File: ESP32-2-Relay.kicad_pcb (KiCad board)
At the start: 2 copper layers, 98 x 94 mm, 44 parts, among them J1 Relay-1, J2 Relay-2, J3 USB_C_Receptacle_USB2.0, K1 SRD-05VDC-SL-C, K2 SRD-05VDC-SL-C, Q1 BC857, Q2 BC857, Q3 BC847W, Q4 BC847W, SW3 SW_Push, SW4 SW_Push, U1 AMS1117-3.3, U4 ESP32-WROOM-32, U5 PC817, U6 PC817, U7 USBLC6-2SC6, U8 CP2102N-Axx-xQFN28

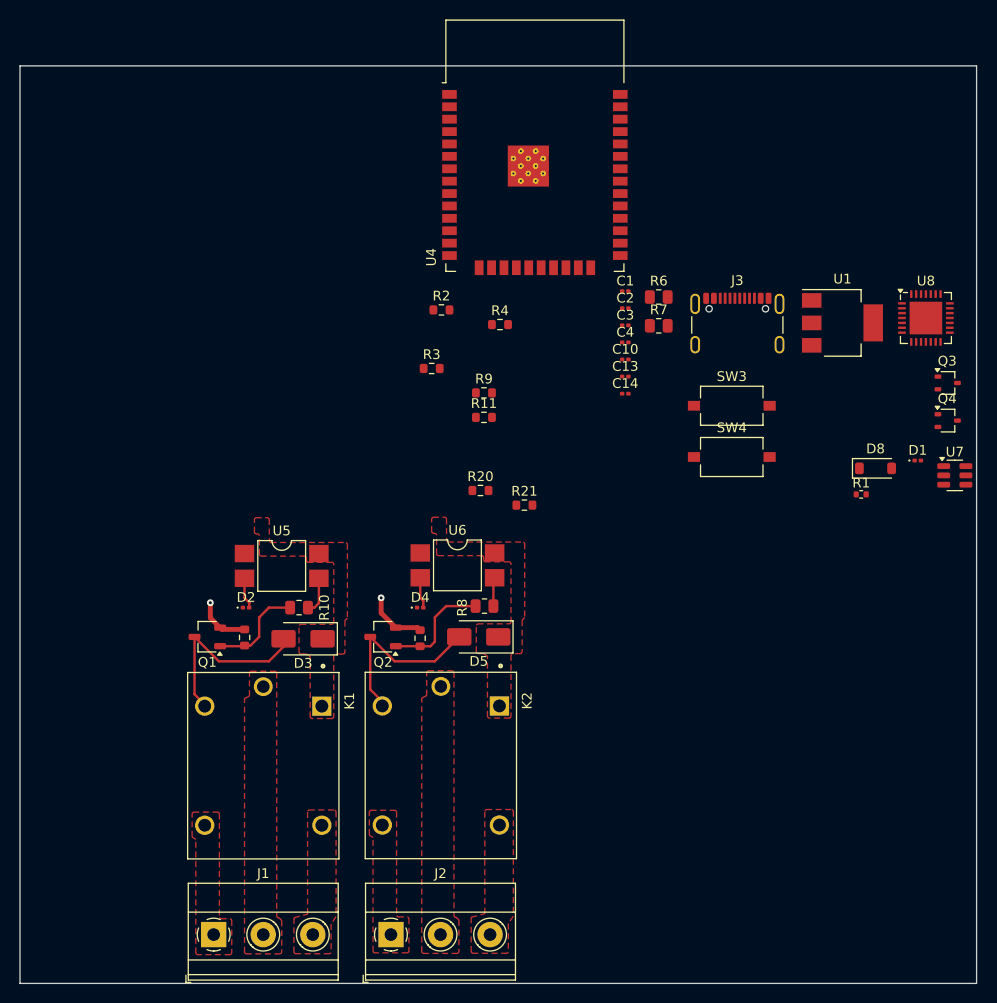
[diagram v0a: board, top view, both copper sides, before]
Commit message: 17h
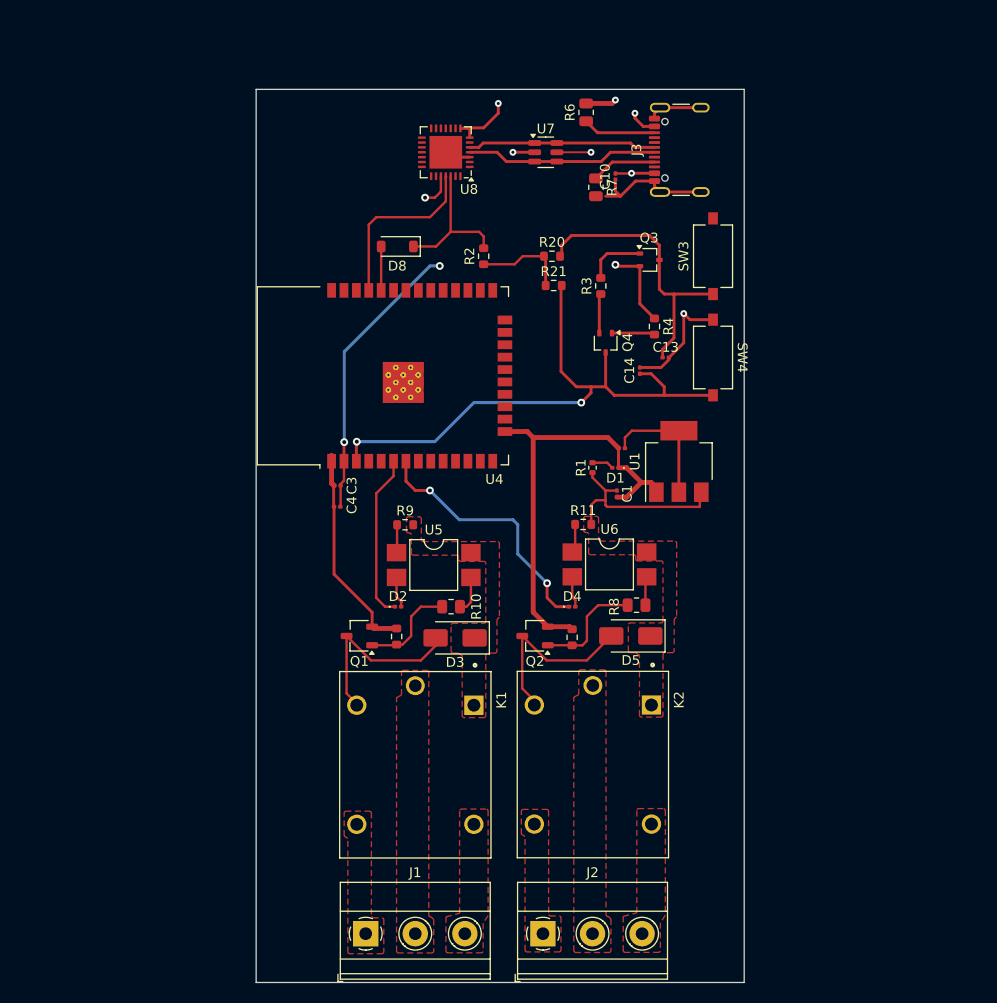
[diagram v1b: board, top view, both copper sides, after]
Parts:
- moved D8 54.0 mm to (173.2, 73.5), turned to 180 degrees
- moved U7 53.4 mm to (188.4, 63.9)
- moved U8 52.0 mm to (178.1, 63.9), turned to 180 degrees
- moved Q4 35.9 mm to (194.5, 83.4), turned to -90 degrees
- moved C4 34.0 mm to (167.0, 100.2), turned to 180 degrees
- moved C3 33.7 mm to (167.0, 98.0), turned to 180 degrees
- moved Q3 33.0 mm to (199.0, 74.9)
- moved D1 31.0 mm to (195.5, 96.2), turned to 180 degrees
- moved R1 27.7 mm to (193.2, 96.2), turned to 90 degrees
- moved R20 25.1 mm to (189.0, 74.5)
- moved U4 24.1 mm to (174.7, 86.8), turned to 90 degrees
- moved R21 22.7 mm to (189.2, 77.5)
- moved U1 22.0 mm to (202.0, 95.5), turned to 90 degrees
- moved C1 20.8 mm to (195.7, 98.8), turned to -90 degrees
- moved R6 20.3 mm to (192.5, 59.8), turned to 90 degrees
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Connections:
- C2 pad 1: +3.3V -> +3V3
- D2 pad 1: /IO_21 -> /IO_34
- D4 pad 1: /IO_19 -> /IO_35
- U1 pad 2: +3.3V -> +3V3
- U4 pad 31: /IO_19 -> unconnected-(U4-IO19-Pad31)
- U4 pad 33: /IO_21 -> unconnected-(U4-IO21-Pad33)
- U4 pad 6: unconnected-(U4-IO34-Pad6) -> /IO_34
- U4 pad 7: unconnected-(U4-IO35-Pad7) -> /IO_35
- U8 pad 1: unconnected-(U8-~{DCD}-Pad1) -> /DTR
- U8 pad 28: /DTR -> unconnected-(U8-~{DTR}-Pad28)
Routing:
- net GND: track 11.8 -> 106.0 mm, vias 2 -> 3
- net /RESET: track 0.00 -> 61.6 mm, vias 0 -> 2
- net +3V3: track 0.00 -> 52.8 mm, vias 0 -> 2
- net +5V: track 0.00 -> 33.4 mm, vias 0 -> 4
- net /BOOT: track 0.00 -> 29.0 mm
- net /IO_35: track 0.00 -> 26.7 mm, vias 0 -> 2
- net /D+: track 0.00 -> 19.7 mm
- net /D-: track 0.00 -> 19.3 mm
- net /RX: track 0.00 -> 18.3 mm
- net /IO_34: track 0.00 -> 17.0 mm
- net /TX: track 0.00 -> 14.9 mm
- net /DTR: track 0.00 -> 8.53 mm, vias 0 -> 1
- net /RTS: track 0.00 -> 7.52 mm, vias 0 -> 1
- net Net-(J3-CC2): track 0.00 -> 7.49 mm
- net Net-(J3-CC1): track 0.00 -> 6.69 mm
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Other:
- board size 98 x 94 mm -> 50 x 91.5 mm

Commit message: done
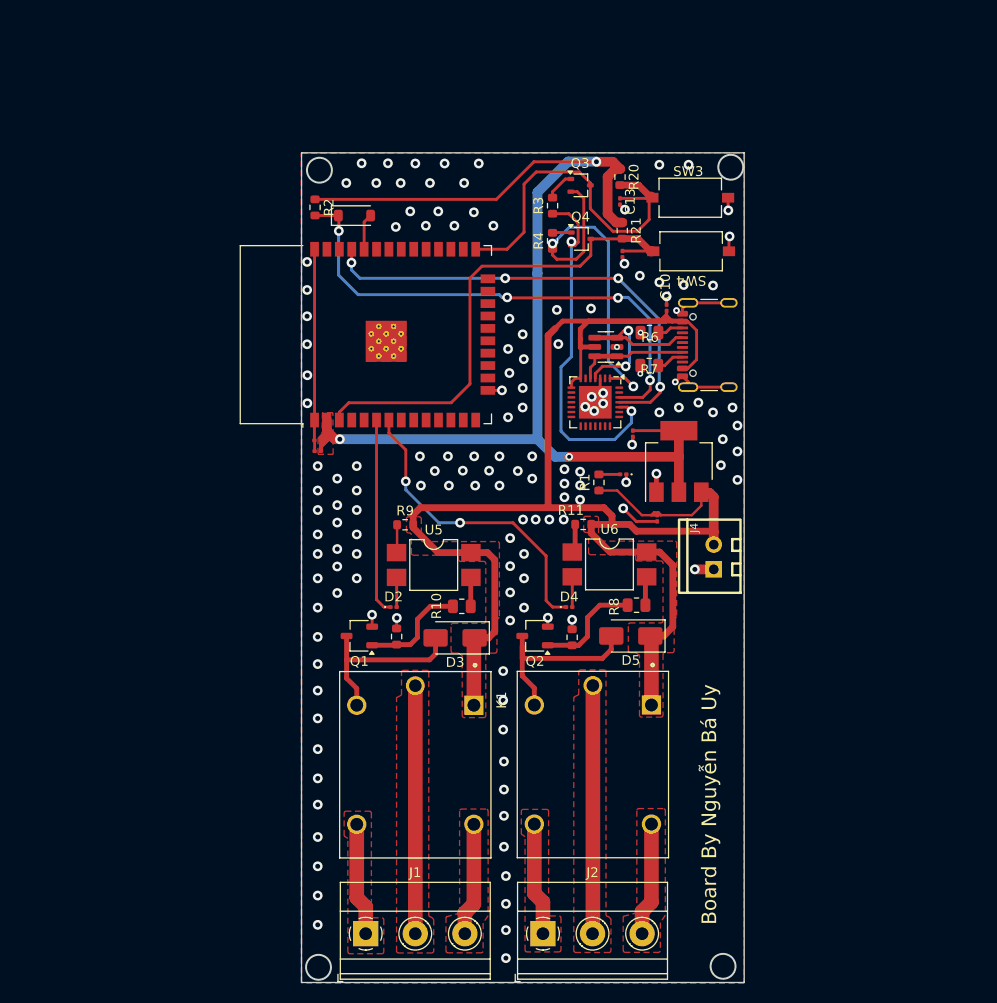
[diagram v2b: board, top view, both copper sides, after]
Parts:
- added J4: Conn_01x02, TRUNGTHAO:Conn_XH-P2.54mm-2P, F.Cu at (205.5, 105.2)
- R1: footprint Resistor_SMD:R_0402_1005Metric -> Resistor_SMD:R_0603_1608Metric
- moved U8 29.8 mm to (193.4, 89.5), turned to -90 degrees
- moved R6 23.5 mm to (199.0, 82.3), turned to 180 degrees
- moved U7 20.9 mm to (194.5, 83.8), turned to 180 degrees
- moved J3 20.2 mm to (206.1, 83.6)
- moved R7 19.1 mm to (199.0, 85.7), turned to 180 degrees
- moved R2 18.0 mm to (164.7, 69.5), turned to -90 degrees
- moved C13 16.7 mm to (196.0, 68.9), turned to -90 degrees
- moved C10 14.4 mm to (200.7, 79.8), turned to -90 degrees
- moved R4 13.6 mm to (189.1, 72.9), turned to 90 degrees
- moved C14 12.1 mm to (196.2, 74.3), turned to -90 degrees
- moved SW4 11.1 mm to (203.3, 74.0), turned to 180 degrees
- moved Q4 10.9 mm to (192.0, 72.7), turned to 0 degrees
- moved R20 10.7 mm to (196.0, 66.4), turned to -90 degrees
- moved Q3 10.4 mm to (191.9, 67.2)
- moved R3 9.60 mm to (189.1, 69.3)
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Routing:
- net +5V: track 33.4 -> 175.2 mm, vias 4 -> 1
- net +3V3: track 52.8 -> 130.5 mm, vias 2 -> 3
- net GND: track 106.0 -> 63.0 mm, vias 3 -> 146
- net /TX: track 14.9 -> 53.1 mm, vias 0 -> 4
- net /RX: track 18.3 -> 47.9 mm, vias 0 -> 4
- net /RTS: track 7.52 -> 36.9 mm, vias 1 -> 2
- net /DTR: track 8.53 -> 37.6 mm, vias 1 -> 2
- net /COM-2: track 0.00 -> 25.4 mm
- net /COM-1: track 0.00 -> 25.4 mm
- net /NC-2: track 0.00 -> 11.6 mm
- net /NC-1: track 0.00 -> 11.6 mm
- net /NO-2: track 0.00 -> 11.6 mm
- net /NO-1: track 0.00 -> 11.6 mm
- net /RESET: track 61.6 -> 51.2 mm, vias 2 -> 0
- net /BOOT: track 29.0 -> 37.7 mm
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- added copper zone on F.Cu, net +3V3
- added copper zone on B.Cu, net GND
- added copper zone on F.Cu, net GND
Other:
- board size 50 x 91.5 mm -> 45.4 x 85 mm
- board text added: "Board By Nguyễn Bá Uy"

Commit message: lastest
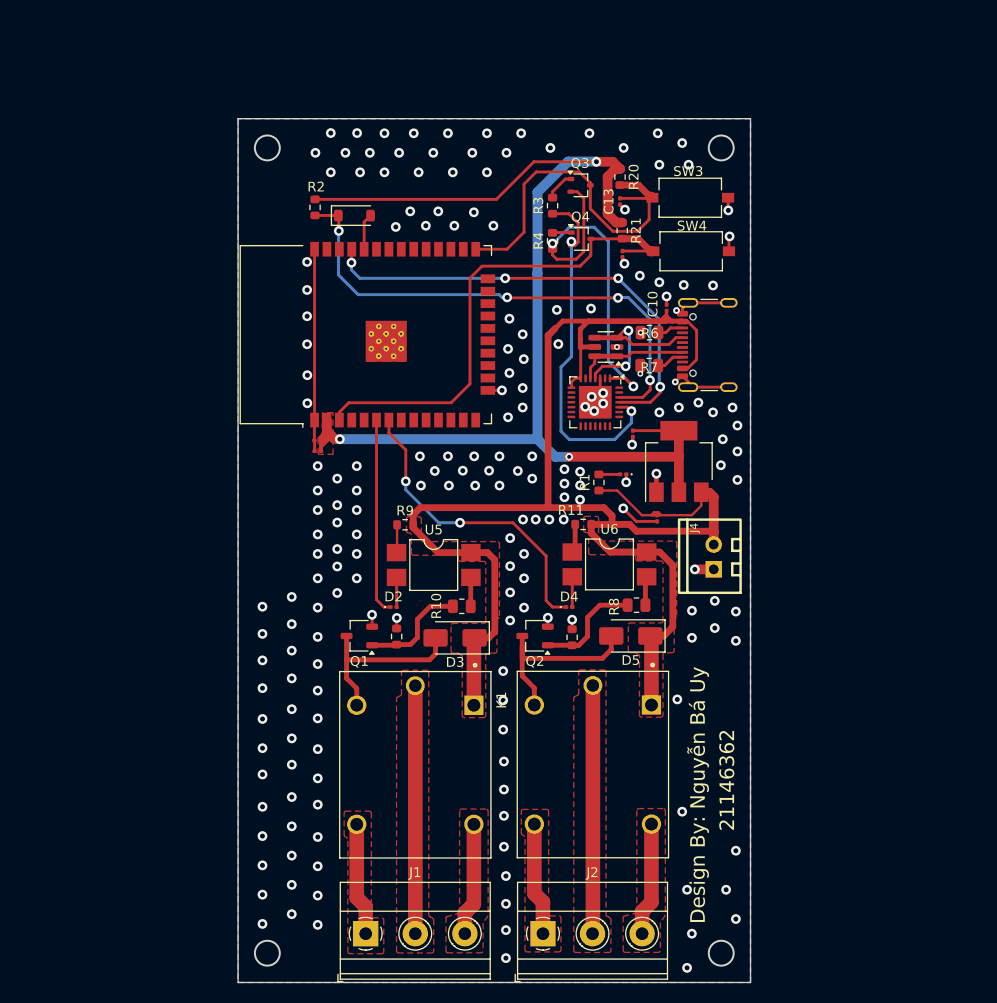
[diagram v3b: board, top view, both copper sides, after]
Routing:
- net GND: track 63.0 -> 63.3 mm, vias 146 -> 199
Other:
- board size 45.4 x 85 mm -> 52.5 x 88.5 mm
- board text added: "21146362"
- board text added: "Design By: Nguyễn Bá Uy"
- board text removed: "Board By Nguyễn Bá Uy"
